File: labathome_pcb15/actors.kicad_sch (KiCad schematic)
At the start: 39 parts, among them J18 K1, J24 K1, J7 FAN5V, J8 GN 5V RGB GN, K1 G6K-2, Q1 BC817, Q2 IRLML6344, Q3 TIP41, Q4 BC817, Q5 IRLML6344, X1 FAN_6024

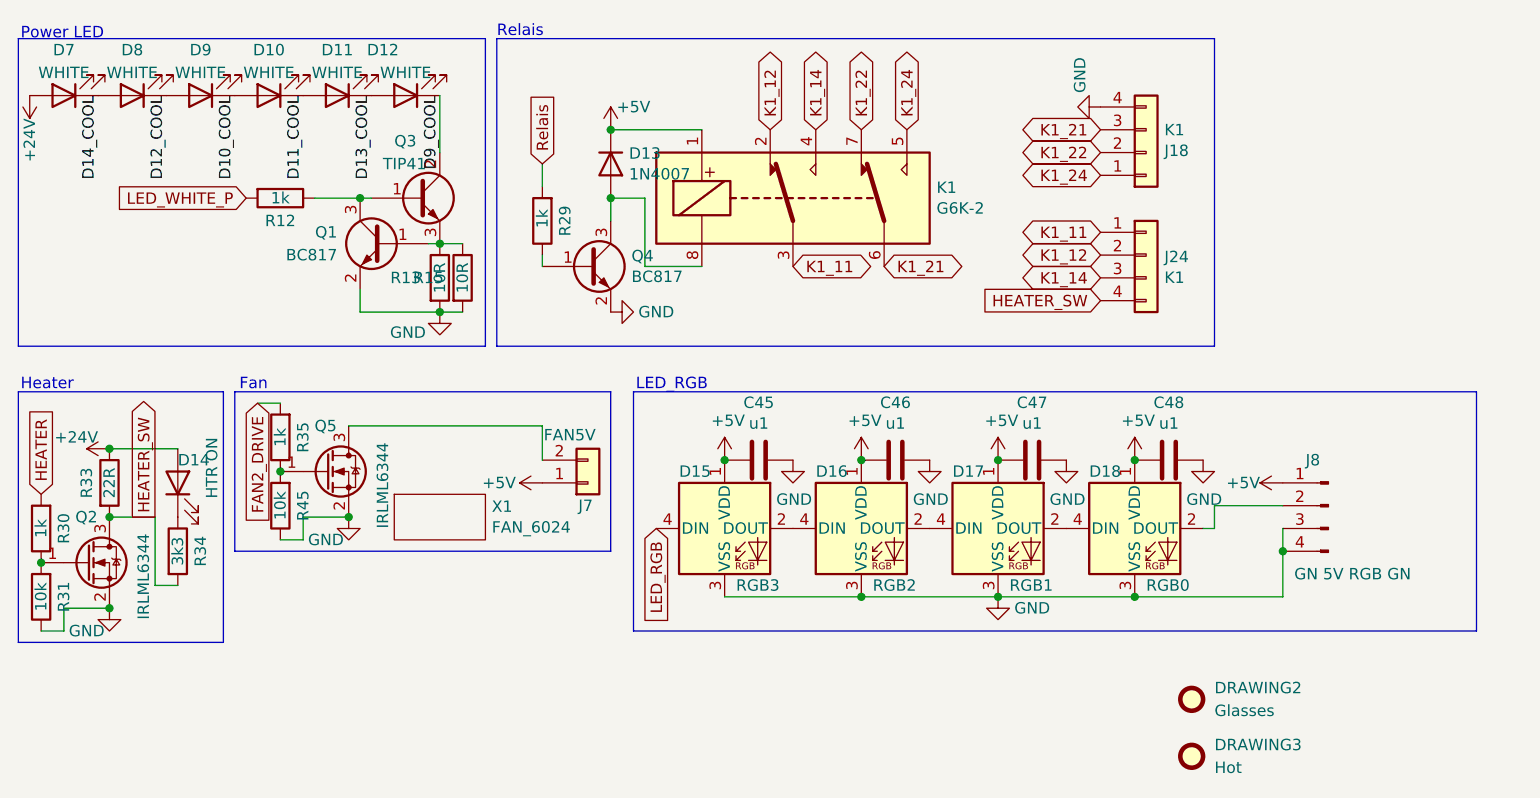
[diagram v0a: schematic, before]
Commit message: labathome_pcb15 ready for first review
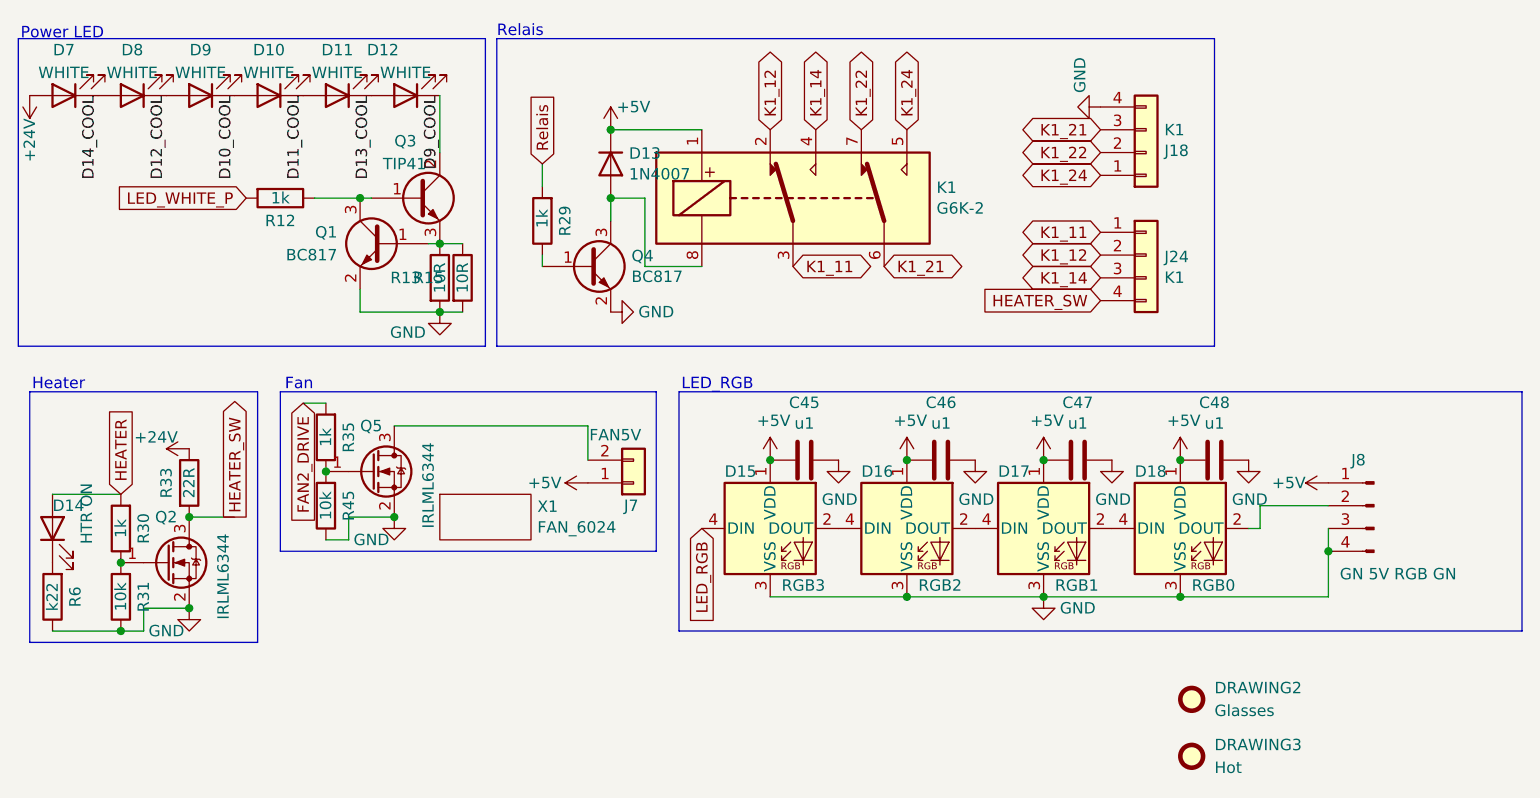
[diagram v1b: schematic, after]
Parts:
- removed R34: 3k3, Resistor_SMD:R_1206_3216Metric, symbol Device:R
- added R6: k22, Resistor_SMD:R_0402_1005Metric, symbol Device:R
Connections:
- net +24V: no longer D14.2 (A)
- net GND: now also R6.1
- net HEATER: now also D14.2 (A)
- net at D14.1 (K): now also R6.2
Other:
- moved on the sheet: C45, C46, C47, C48, D14, D15, D16, D17, D18, J7, J8, Q2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
